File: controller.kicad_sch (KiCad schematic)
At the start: 24 parts, among them U1 nRF52840, X1 32MHz, X2 32.768kHz

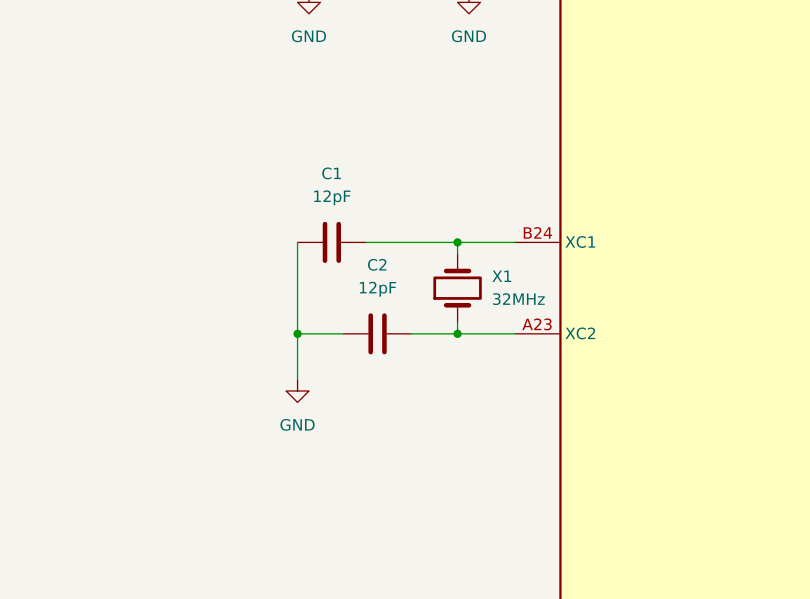
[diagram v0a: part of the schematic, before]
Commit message: first jlc submission
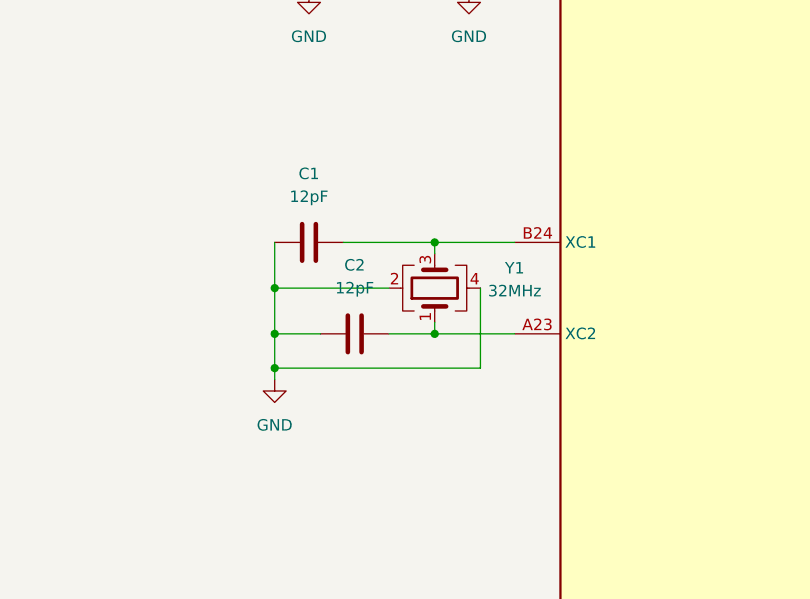
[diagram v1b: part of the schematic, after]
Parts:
- removed X1: 32MHz, Crystal:Crystal_SMD_0603-2Pin_6.0x3.5mm, symbol Device:Crystal
- added Y1: 32MHz, Crystal:Crystal_SMD_2016-4Pin_2.0x1.6mm, symbol Device:Crystal_GND24
- X2: LCSC (none) -> C182057
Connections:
- net GND: now also Y1.2, Y1.4
- net at C2.2, U1.A23 (XC2): now also Y1.1
- net at C1.2, U1.B24 (XC1): now also Y1.3
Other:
- moved on the sheet: C1, C2
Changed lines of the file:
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@@
   (junction (at 102.87 38.1) (diameter 0) (color 0 0 0 0)
   )
-  (junction (at 54.61 123.19) (diameter 0) (color 0 0 0 0)
+  (junction (at 52.07 123.19) (diameter 0) (color 0 0 0 0)
   )
   (junction (at 59.69 57.15) (diameter 0) (color 0 0 0 0)
@@
   (junction (at 73.66 72.39) (diameter 0) (color 0 0 0 0)
   )
-  (junction (at 72.39 113.03) (diameter 0) (color 0 0 0 0)
+  (junction (at 69.85 113.03) (diameter 0) (color 0 0 0 0)
+  )
+  (junction (at 52.07 127) (diameter 0) (color 0 0 0 0)
   )
   (junction (at 149.86 36.83) (diameter 0) (color 0 0 0 0)
@@
   (junction (at 55.88 72.39) (diameter 0) (color 0 0 0 0)
   )
-  (junction (at 72.39 123.19) (diameter 0) (color 0 0 0 0)
+  (junction (at 69.85 123.19) (diameter 0) (color 0 0 0 0)
   )
   (junction (at 72.39 57.15) (diameter 0) (color 0 0 0 0)
@@
   (junction (at 77.47 27.94) (diameter 0) (color 0 0 0 0)
   )
+  (junction (at 52.07 118.11) (diameter 0) (color 0 0 0 0)
+  )
   (wire (pts (xy 90.17 27.94) (xy 90.17 29.21))
     (stroke (width 0) (type default))
@@
     (stroke (width 0) (type default))
   )
-  (wire (pts (xy 72.39 113.03) (xy 78.74 113.03))
+  (wire (pts (xy 69.85 113.03) (xy 78.74 113.03))
     (stroke (width 0) (type default))
   )
@@
     (stroke (width 0) (type default))
   )
+  (wire (pts (xy 52.07 118.11) (xy 52.07 123.19))
+    (stroke (width 0) (type default))
+  )
+  (wire (pts (xy 52.07 118.11) (xy 64.77 118.11))
+    (stroke (width 0) (type default))
+  )
   (wire (pts (xy 101.6 46.99) (xy 101.6 44.45))
     (stroke (width 0) (type default))
@@
     (stroke (width 0) (type default))
   )
+  (wire (pts (xy 74.93 127) (xy 74.93 118.11))
+    (stroke (width 0) (type default))
+  )
   (wire (pts (xy 64.77 36.83) (xy 64.77 38.1))
     (stroke (width 0) (type default))
@@
     (stroke (width 0) (type default))
   )
+  (wire (pts (xy 52.07 127) (xy 74.93 127))
+    (stroke (width 0) (type default))
+  )
   (wire (pts (xy 46.99 44.45) (xy 46.99 46.99))
     (stroke (width 0) (type default))
@@
     (stroke (width 0) (type default))
   )
-  (wire (pts (xy 72.39 113.03) (xy 72.39 114.3))
+  (wire (pts (xy 69.85 113.03) (xy 69.85 114.3))
     (stroke (width 0) (type default))
   )
@@
     (stroke (width 0) (type default))
   )
-  (wire (pts (xy 54.61 123.19) (xy 54.61 128.27))
-    (stroke (width 0) (type default))
-  )
-  (wire (pts (xy 67.31 123.19) (xy 72.39 123.19))
+  (wire (pts (xy 52.07 123.19) (xy 52.07 127))
+    (stroke (width 0) (type default))
+  )
+  (wire (pts (xy 64.77 123.19) (xy 69.85 123.19))
     (stroke (width 0) (type default))
   )
@@
     (stroke (width 0) (type default))
   )
-  (wire (pts (xy 54.61 123.19) (xy 59.69 123.19))
+  (wire (pts (xy 52.07 123.19) (xy 57.15 123.19))
     (stroke (width 0) (type default))
   )
@@
     (stroke (width 0) (type default))
   )
-  (wire (pts (xy 54.61 113.03) (xy 54.61 123.19))
+  (wire (pts (xy 52.07 113.03) (xy 52.07 118.11))
     (stroke (width 0) (type default))
   )
@@
     (stroke (width 0) (type default))
   )
-  (wire (pts (xy 62.23 113.03) (xy 72.39 113.03))
+  (wire (pts (xy 59.69 113.03) (xy 69.85 113.03))
     (stroke (width 0) (type default))
   )
@@
     (stroke (width 0) (type default))
   )
-  (wire (pts (xy 72.39 123.19) (xy 78.74 123.19))
+  (wire (pts (xy 69.85 123.19) (xy 78.74 123.19))
     (stroke (width 0) (type default))
   )
@@
     (stroke (width 0) (type default))
   )
-  (wire (pts (xy 72.39 121.92) (xy 72.39 123.19))
+  (wire (pts (xy 52.07 127) (xy 52.07 128.27))
+    (stroke (width 0) (type default))
+  )
+  (wire (pts (xy 69.85 121.92) (xy 69.85 123.19))
     (stroke (width 0) (type default))
   )
@@
     )
   )
+  (symbol (lib_id "Device:Crystal_GND24") (at 69.85 118.11 90) (unit 1)
+    (in_bom yes) (on_board yes) (dnp no) (fields_autoplaced)
+    (property "Reference" "Y1" (at 78.74 115.8941 90)
+      (effects (font (size 1.27 1.27)))
+    )
+    (property "Value" "32MHz" (at 78.74 118.4341 90)
+      (effects (font (size 1.27 1.27)))
+    )
+    (property "Footprint" "Crystal:Crystal_SMD_2016-4Pin_2.0x1.6mm" (at 69.85 118.11 0)
+      (effects (font (size 1.27 1.27)) hide)
+    )
+    (property "Datasheet" "~" (at 69.85 118.11 0)
+      (effects (font (size 1.27 1.27)) hide)
+    )
+    (property "LCSC" "C2965582" (at 69.85 118.11 90)
+      (effects (font (size 1.27 1.27)) hide)
+    )
+    (pin "2")
+    (pin "1")
+    (pin "4")
+    (pin "3")
+    (instances
+      (project "keyboard"
+        (path "/a3795772-e8b2-4a24-8aa0-5a93e6e5ac56/824037f1-2051-4dfb-9b54-5b5661939278"
+          (reference "Y1") (unit 1)
+        )
+      )
+    )
+  )
   (symbol (lib_id "Device:C") (at 59.69 50.8 0) (unit 1)
     (in_bom yes) (on_board yes) (dnp no) (fields_autoplaced)
@@
     )
   )
-  (symbol (lib_id "Device:Crystal") (at 72.39 118.11 90) (unit 1)
-    (in_bom yes) (on_board yes) (dnp no) (fields_autoplaced)
-    (property "Reference" "X1" (at 76.2 116.84 90)
-      (effects (font (size 1.27 1.27)) (justify right))
-    )
-    (property "Value" "32MHz" (at 76.2 119.38 90)
-      (effects (font (size 1.27 1.27)) (justify right))
-    )
-    (property "Footprint" "Crystal:Crystal_SMD_0603-2Pin_6.0x3.5mm" (at 72.39 118.11 0)
-      (effects (font (size 1.27 1.27)) hide)
-    )
-    (property "Datasheet" "~" (at 72.39 118.11 0)
-      (effects (font (size 1.27 1.27)) hide)
-    )
-    (pin "1")
-    (pin "2")
-    (instances
-      (project "keyboard"
-        (path "/a3795772-e8b2-4a24-8aa0-5a93e6e5ac56/824037f1-2051-4dfb-9b54-5b5661939278"
-          (reference "X1") (unit 1)
-        )
-      )
-    )
-  )
   (symbol (lib_id "Device:Crystal") (at 149.86 41.91 90) (unit 1)
     (in_bom yes) (on_board yes) (dnp no) (fields_autoplaced)
@@
       (effects (font (size 1.27 1.27)) hide)
     )
+    (property "LCSC" "C182057" (at 149.86 41.91 90)
+      (effects (font (size 1.27 1.27)) hide)
+    )
     (pin "2")
     (pin "1")
@@
     )
   )
-  (symbol (lib_id "power:GND") (at 54.61 128.27 0) (unit 1)
-    (in_bom yes) (on_board yes) (dnp no) (fields_autoplaced)
-    (property "Reference" "#PWR03" (at 54.61 134.62 0)
-      (effects (font (size 1.27 1.27)) hide)
-    )
-    (property "Value" "GND" (at 54.61 133.35 0)
-      (effects (font (size 1.27 1.27)))
-    )
-    (property "Footprint" "" (at 54.61 128.27 0)
-      (effects (font (size 1.27 1.27)) hide)
-    )
-    (property "Datasheet" "" (at 54.61 128.27 0)
+  (symbol (lib_id "power:GND") (at 52.07 128.27 0) (unit 1)
+    (in_bom yes) (on_board yes) (dnp no) (fields_autoplaced)
+    (property "Reference" "#PWR03" (at 52.07 134.62 0)
+      (effects (font (size 1.27 1.27)) hide)
+    )
+    (property "Value" "GND" (at 52.07 133.35 0)
+      (effects (font (size 1.27 1.27)))
+    )
+    (property "Footprint" "" (at 52.07 128.27 0)
+      (effects (font (size 1.27 1.27)) hide)
+    )
+    (property "Datasheet" "" (at 52.07 128.27 0)
       (effects (font (size 1.27 1.27)) hide)
     )
@@
     )
   )
-  (symbol (lib_id "Device:C") (at 58.42 113.03 90) (unit 1)
-    (in_bom yes) (on_board yes) (dnp no) (fields_autoplaced)
-    (property "Reference" "C1" (at 58.42 105.41 90)
-      (effects (font (size 1.27 1.27)))
-    )
-    (property "Value" "12pF" (at 58.42 107.95 90)
-      (effects (font (size 1.27 1.27)))
-    )
-    (property "Footprint" "Capacitor_SMD:C_0603_1608Metric" (at 62.23 112.0648 0)
-      (effects (font (size 1.27 1.27)) hide)
-    )
-    (property "Datasheet" "~" (at 58.42 113.03 0)
+  (symbol (lib_id "Device:C") (at 55.88 113.03 90) (unit 1)
+    (in_bom yes) (on_board yes) (dnp no) (fields_autoplaced)
+    (property "Reference" "C1" (at 55.88 105.41 90)
+      (effects (font (size 1.27 1.27)))
+    )
+    (property "Value" "12pF" (at 55.88 107.95 90)
+      (effects (font (size 1.27 1.27)))
+    )
+    (property "Footprint" "Capacitor_SMD:C_0603_1608Metric" (at 59.69 112.0648 0)
+      (effects (font (size 1.27 1.27)) hide)
+    )
+    (property "Datasheet" "~" (at 55.88 113.03 0)
       (effects (font (size 1.27 1.27)) hide)
     )
@@
     )
   )
-  (symbol (lib_id "Device:C") (at 63.5 123.19 90) (unit 1)
-    (in_bom yes) (on_board yes) (dnp no) (fields_autoplaced)
-    (property "Reference" "C2" (at 63.5 115.57 90)
-      (effects (font (size 1.27 1.27)))
-    )
-    (property "Value" "12pF" (at 63.5 118.11 90)
-      (effects (font (size 1.27 1.27)))
-    )
-    (property "Footprint" "Capacitor_SMD:C_0603_1608Metric" (at 67.31 122.2248 0)
-      (effects (font (size 1.27 1.27)) hide)
-    )
-    (property "Datasheet" "~" (at 63.5 123.19 0)
-      (effects (font (size 1.27 1.27)) hide)
-    )
+  (symbol (lib_id "Device:C") (at 60.96 123.19 90) (unit 1)
+    (in_bom yes) (on_board yes) (dnp no) (fields_autoplaced)
+    (property "Reference" "C2" (at 60.96 115.57 90)
+      (effects (font (size 1.27 1.27)))
+    )
+    (property "Value" "12pF" (at 60.96 118.11 90)
+      (effects (font (size 1.27 1.27)))
+    )
+    (property "Footprint" "Capacitor_SMD:C_0603_1608Metric" (at 64.77 122.2248 0)
+      (effects (font (size 1.27 1.27)) hide)
+    )
+    (property "Datasheet" "~" (at 60.96 123.19 0)
+      (effects (font (size 1.27 1.27)) hide)
+    )
